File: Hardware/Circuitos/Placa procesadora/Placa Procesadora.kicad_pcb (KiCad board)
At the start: 2 copper layers, 46 x 45 mm, 26 parts, among them J1 Conn_01x02, J2 Conn_01x02, J7 Conn_01x02, U1 LM358

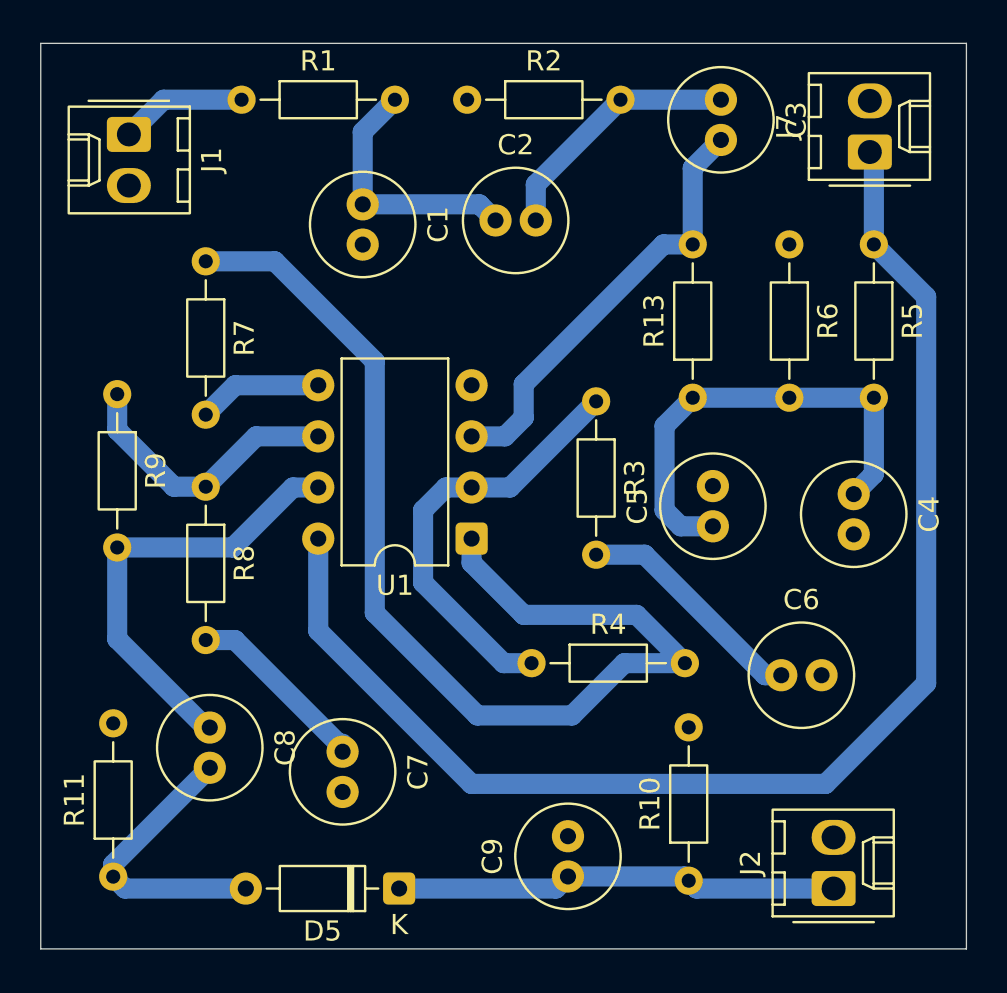
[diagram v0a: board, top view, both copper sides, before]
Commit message: Placa procesadora - Zona de tierra PCB
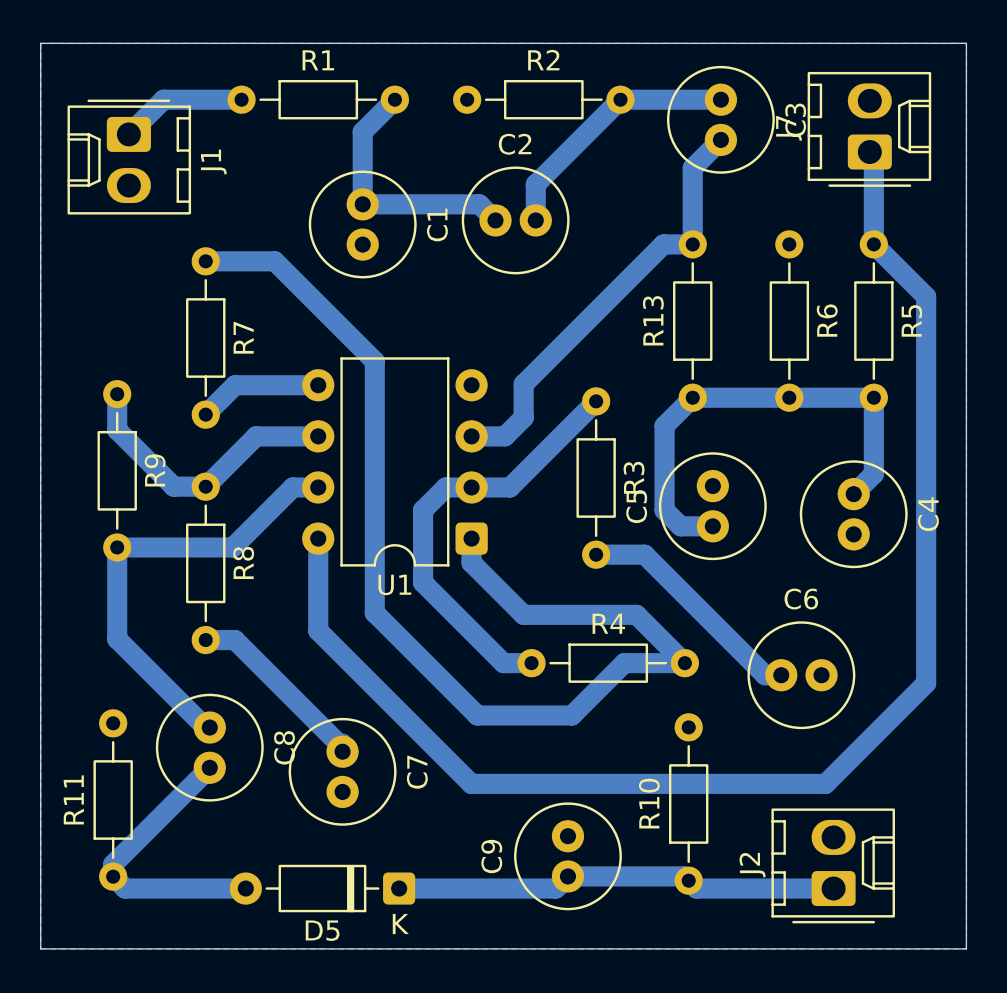
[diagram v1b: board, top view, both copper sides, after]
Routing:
- added copper zone on B.Cu, net Earth
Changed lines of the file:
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@@
 		(net "Net-(U1B-+)")
+	)
+	(zone
+		(net "Earth")
+		(layer "B.Cu")
+		(hatch edge 0.5)
+		(connect_pads
+			(clearance 0.5)
+		)
+		(min_thickness 0.25)
+		(fill yes
+			(thermal_gap 0.5)
+			(thermal_bridge_width 0.5)
+			(island_removal_mode 0)
+		)
+		(polygon
+			(pts
+				(xy 157 34.8) (xy 111 34.8) (xy 111 79.8) (xy 157 79.8)
+			)
+		)
 	)
 	(embedded_fonts no)
